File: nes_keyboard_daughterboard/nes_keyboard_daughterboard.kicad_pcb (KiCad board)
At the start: 4 copper layers, 77.2 x 44 mm, 74 parts, among them J1 USB_C_Receptacle_USB2.0_16P, J2 Conn_01x02_Pin, J3 USB_C_Receptacle_USB2.0_16P, U1 NCP1117-3.3_SOT223, U2 USBLC6-2P6

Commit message: Finished V0.1
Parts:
- D1: value White -> Red
- D2: value Orange -> Red
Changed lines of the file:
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@@
 		(sheetname "/")
 		(sheetfile "nes_keyboard_daughterboard.kicad_sch")
+		(units
+			(unit
+				(name "A")
+				(pins "S1" "B1" "B12" "A1" "A12" "A9" "B4" "B9" "A4" "A5" "B5" "A7" "B7"
+					"A6" "B6" "A8" "B8"
+				)
+			)
+		)
 		(attr smd)
 		(duplicate_pad_numbers_are_jumpers no)
@@
 		(sheetname "/")
 		(sheetfile "nes_keyboard_daughterboard.kicad_sch")
+		(units
+			(unit
+				(name "A")
+				(pins "1" "2")
+			)
+		)
 		(attr smd)
 		(duplicate_pad_numbers_are_jumpers no)
@@
 		(sheetname "/")
 		(sheetfile "nes_keyboard_daughterboard.kicad_sch")
+		(units
+			(unit
+				(name "A")
+				(pins "1" "2")
+			)
+		)
 		(attr smd)
 		(duplicate_pad_numbers_are_jumpers no)
@@
 			)
 		)
-		(property "Value" "Orange"
+		(property "Value" "Red"
 			(at 0 1.43 90)
 			(layer "F.Fab")
@@
 		(sheetname "/")
 		(sheetfile "nes_keyboard_daughterboard.kicad_sch")
+		(units
+			(unit
+				(name "A")
+				(pins "1" "2")
+			)
+		)
 		(attr smd)
 		(duplicate_pad_numbers_are_jumpers no)
@@
 		(sheetname "/")
 		(sheetfile "nes_keyboard_daughterboard.kicad_sch")
+		(units
+			(unit
+				(name "A")
+				(pins "1" "2")
+			)
+		)
 		(attr smd)
 		(duplicate_pad_numbers_are_jumpers no)
@@
 			)
 		)
+		(property "Sim.Library" "/home/arya/Downloads/NCP1117 PSPICE MODELS/NCP1117 Model Library.lib"
+			(at 0 0 270)
+			(unlocked yes)
+			(layer "F.Fab")
+			(hide yes)
+			(effects
+				(font
+					(size 1 1)
+					(thickness 0.15)
+				)
+			)
+		)
+		(property "Sim.Name" "ncp1117_33-x"
+			(at 0 0 270)
+			(unlocked yes)
+			(layer "F.Fab")
+			(hide yes)
+			(effects
+				(font
+					(size 1 1)
+					(thickness 0.15)
+				)
+			)
+		)
+		(property "Sim.Device" "SUBCKT"
+			(at 0 0 270)
+			(unlocked yes)
+			(layer "F.Fab")
+			(hide yes)
+			(effects
+				(font
+					(size 1 1)
+					(thickness 0.15)
+				)
+			)
+		)
+		(property "Sim.Pins" "1=1 2=2 3=3"
+			(at 0 0 270)
+			(unlocked yes)
+			(layer "F.Fab")
+			(hide yes)
+			(effects
+				(font
+					(size 1 1)
+					(thickness 0.15)
+				)
+			)
+		)
 		(property ki_fp_filters "SOT?223*TabPin2*")
 		(sheetname "/")
 		(sheetfile "nes_keyboard_daughterboard.kicad_sch")
+		(units
+			(unit
+				(name "A")
+				(pins "3" "1" "2")
+			)
+		)
 		(attr smd)
 		(duplicate_pad_numbers_are_jumpers no)
@@
 			)
 		)
-		(property "Value" "White"
+		(property "Value" "Red"
 			(at 0 1.43 90)
 			(layer "F.Fab")
@@
 			)
 		)
-		(property "Sim.Pins" "1=K 2=A"
+		(property "Sim.Pins" "1=A 2=K"
+			(at 0 0 270)
+			(unlocked yes)
+			(layer "F.Fab")
+			(hide yes)
+			(effects
+				(font
+					(size 1 1)
+					(thickness 0.15)
+				)
+			)
+		)
+		(property "Sim.Device" "D"
+			(at 0 0 270)
+			(unlocked yes)
+			(layer "F.Fab")
+			(hide yes)
+			(effects
+				(font
+					(size 1 1)
+					(thickness 0.15)
+				)
+			)
+		)
+		(property "Sim.Params" "is=0.03 vj=2 bv=5 ibv=0.0001"
 			(at 0 0 270)
 			(unlocked yes)
@@
 		(sheetname "/")
 		(sheetfile "nes_keyboard_daughterboard.kicad_sch")
+		(units
+			(unit
+				(name "A")
+				(pins "1" "2")
+			)
+		)
 		(attr smd)
 		(duplicate_pad_numbers_are_jumpers no)
@@
 		(sheetname "/")
 		(sheetfile "nes_keyboard_daughterboard.kicad_sch")
+		(units
+			(unit
+				(name "A")
+				(pins "1")
+			)
+		)
 		(attr exclude_from_bom)
 		(duplicate_pad_numbers_are_jumpers no)
@@
 		(sheetname "/")
 		(sheetfile "nes_keyboard_daughterboard.kicad_sch")
+		(units
+			(unit
+				(name "A")
+				(pins "1" "3" "5" "2" "6" "4")
+			)
+		)
 		(attr smd)
 		(duplicate_pad_numbers_are_jumpers no)
@@
 		(sheetname "/")
 		(sheetfile "nes_keyboard_daughterboard.kicad_sch")
+		(units
+			(unit
+				(name "A")
+				(pins "1" "2")
+			)
+		)
 		(attr smd)
 		(duplicate_pad_numbers_are_jumpers no)
@@
 		(sheetname "/")
 		(sheetfile "nes_keyboard_daughterboard.kicad_sch")
+		(units
+			(unit
+				(name "A")
+				(pins "S1" "B1" "B12" "A1" "A12" "A9" "B4" "B9" "A4" "A5" "B5" "A7" "B7"
+					"A6" "B6" "A8" "B8"
+				)
+			)
+		)
 		(attr through_hole)
 		(duplicate_pad_numbers_are_jumpers no)
@@
 		(sheetname "/")
 		(sheetfile "nes_keyboard_daughterboard.kicad_sch")
+		(units
+			(unit
+				(name "A")
+				(pins "1" "2")
+			)
+		)
 		(attr smd)
 		(duplicate_pad_numbers_are_jumpers no)
@@
 		(sheetname "/")
 		(sheetfile "nes_keyboard_daughterboard.kicad_sch")
+		(units
+			(unit
+				(name "A")
+				(pins "1")
+			)
+		)
 		(attr exclude_from_bom)
 		(duplicate_pad_numbers_are_jumpers no)
@@
 		(sheetname "/")
 		(sheetfile "nes_keyboard_daughterboard.kicad_sch")
+		(units
+			(unit
+				(name "A")
+				(pins "1" "2")
+			)
+		)
 		(attr through_hole)
 		(duplicate_pad_numbers_are_jumpers no)
@@
 		(sheetname "/")
 		(sheetfile "nes_keyboard_daughterboard.kicad_sch")
+		(units
+			(unit
+				(name "A")
+				(pins "1" "2")
+			)
+		)
 		(attr smd)
 		(duplicate_pad_numbers_are_jumpers no)
@@
 		(sheetname "/")
 		(sheetfile "nes_keyboard_daughterboard.kicad_sch")
+		(units
+			(unit
+				(name "A")
+				(pins "1")
+			)
+		)
 		(attr exclude_from_bom)
 		(duplicate_pad_numbers_are_jumpers no)
@@
 		(sheetname "/")
 		(sheetfile "nes_keyboard_daughterboard.kicad_sch")
+		(units
+			(unit
+				(name "A")
+				(pins "1")
+			)
+		)
 		(attr exclude_from_bom)
 		(duplicate_pad_numbers_are_jumpers no)

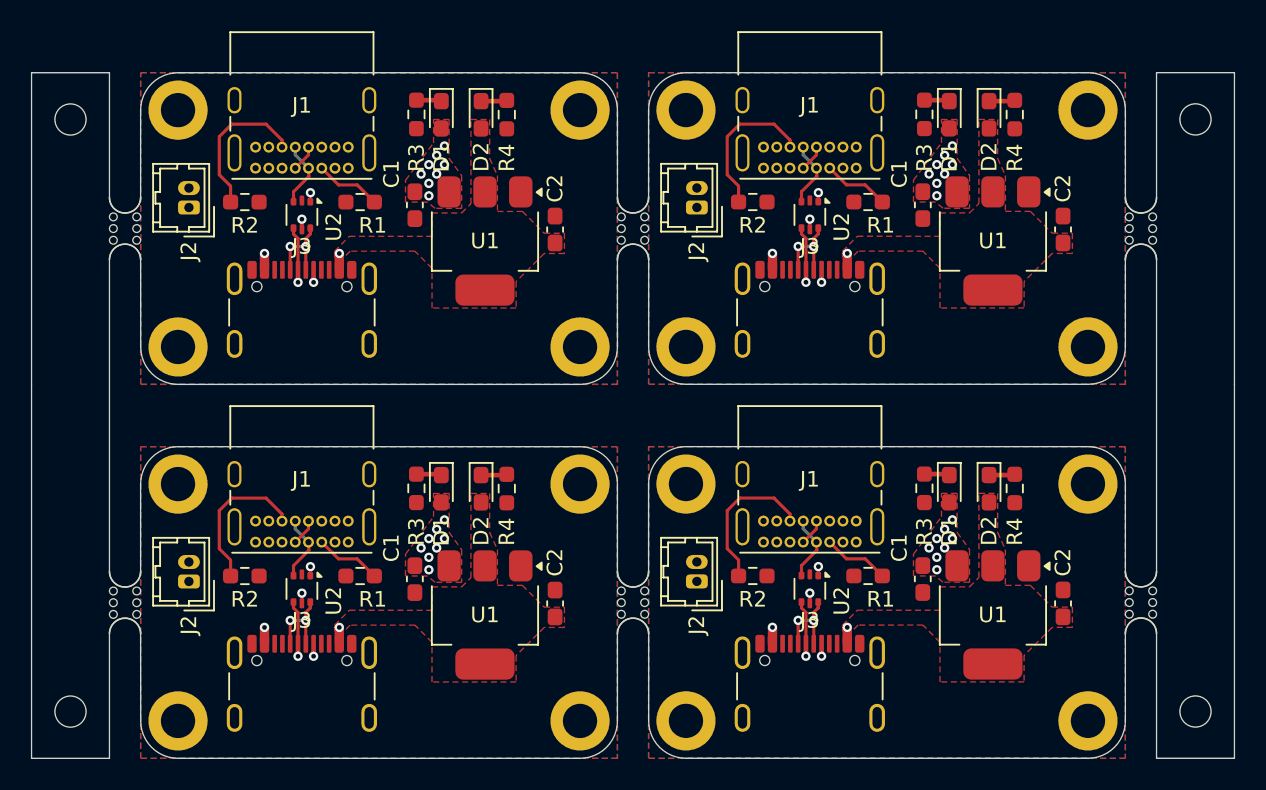
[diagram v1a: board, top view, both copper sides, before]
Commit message: PCB Modifications (all) - V0.2
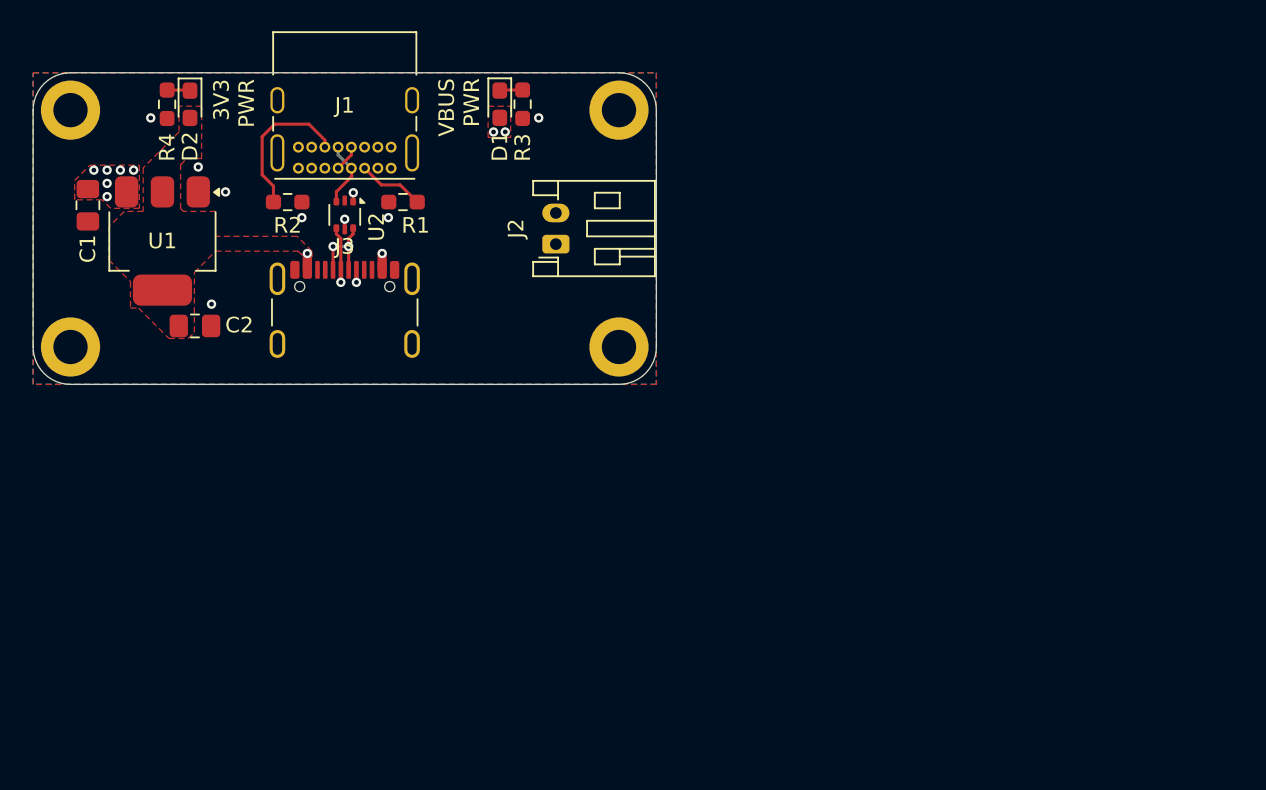
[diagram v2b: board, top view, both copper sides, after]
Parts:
- removed the C1 at (75.1, 28.2)
- removed the C1 at (42.5, 52.2)
- removed the C1 at (75.1, 52.2)
- removed the C1 at (42.5, 28.2)
- removed the C2 at (51.5, 53.8)
- removed the C2 at (84.1, 53.8)
- removed the C2 at (51.5, 29.8)
- removed the C2 at (84.1, 29.8)
- removed the D1 at (76.8, 22.4)
- removed the D1 at (76.8, 46.4)
- removed the D1 at (44.2, 46.4)
- removed the D2 at (46.8, 46.4)
- removed the D2 at (79.4, 22.4)
- removed the D2 at (79.3, 46.4)
- removed the H1 at (27.3, 46.1)
- removed the H1 at (59.9, 22.1)
- removed the H1 at (59.9, 46.1)
- removed the H2 at (59.9, 61.3)
- removed the H2 at (59.9, 37.3)
- removed the H2 at (27.3, 61.3)
- removed the H3 at (85.7, 22.1)
- removed the H3 at (53.1, 46.1)
- removed the H3 at (85.7, 46.1)
- removed the H4 at (85.7, 61.3)
- removed the H4 at (85.7, 37.3)
- removed the H4 at (53.1, 61.3)
- removed the J1 at (70.8, 49.8)
- removed the J1 at (70.8, 25.8)
- removed the J1 at (38.2, 49.8)
- removed the J2 at (28.0, 52.3)
- removed the J2 at (60.6, 52.3)
- removed the J2 at (60.6, 28.3)
- removed the J3 at (67.8, 60.0)
- removed the J3 at (35.2, 60.0)
- removed the J3 at (67.9, 36.0)
- removed the R1 at (71.6, 52.0)
- removed the R1 at (71.6, 28.0)
- removed the R1 at (39.0, 52.0)
- removed the R2 at (64.2, 52.0)
- removed the R2 at (64.2, 28.0)
- removed the R2 at (31.6, 52.0)
- removed the R3 at (42.6, 46.4)
- removed the R3 at (75.2, 46.4)
- removed the R3 at (75.2, 22.4)
- removed the R4 at (81.0, 46.4)
- removed the R4 at (48.4, 46.4)
- removed the R4 at (81.0, 22.4)
- removed the U1 at (79.6, 54.5)
- removed the U1 at (79.6, 30.5)
- removed the U1 at (47.0, 54.5)
- removed the U2 at (67.8, 52.8)
- removed the U2 at (67.9, 28.8)
- removed the U2 at (35.2, 52.8)
- removed mouse-bite-2mm-slot (x6): VAL**, mouse-bite:mouse-bite-2mm-slot
- added C1: 10uF, Capacitor_SMD:C_0805_2012Metric_Pad1.18x1.45mm_HandSolder, F.Cu at (21.5, 28.2)
- added C2: 10uF, Capacitor_SMD:C_0805_2012Metric_Pad1.18x1.45mm_HandSolder, F.Cu at (28.4, 36.0)
- D1: value White -> Red
- D2: value Orange -> Red
- J2: footprint Connector_Hirose:Hirose_DF13-02P-1.25DSA_1x02_P1.25mm_Vertical -> Connector_JST:JST_PH_S2B-PH-K_1x02_P2.00mm_Horizontal
- R3: value 220 -> 680
- R4: value 130 -> 470
- moved J2 23.7 mm to (51.5, 30.7)
- moved R4 21.8 mm to (26.6, 21.7)
- moved U1 20.7 mm to (26.3, 30.5)
- moved D2 18.7 mm to (28.1, 21.7)
- moved H1 6.90 mm to (20.4, 22.1)
- moved H2 6.90 mm to (20.4, 37.3)
- moved R3 6.85 mm to (49.4, 21.7)
- moved D1 3.81 mm to (48.0, 21.7)
- moved J1 2.75 mm to (41.0, 25.8)
- moved J3 2.75 mm to (38.0, 36.0)
- moved R1 2.75 mm to (41.7, 28.0)
- moved R2 2.75 mm to (34.3, 28.0)
- moved U2 2.75 mm to (38.0, 28.8)
- moved H3 2.50 mm to (55.6, 22.1)
- moved H4 2.50 mm to (55.6, 37.3)
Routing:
- net Net-(J1-CC2): track 38.9 -> 9.73 mm
- net +3V3: track 29.9 -> 7.48 mm, vias 8 -> 2
- net /USB_D+: track 22.1 -> 5.52 mm, vias 8 -> 2
- net /USB_D-: track 21.2 -> 5.29 mm, vias 8 -> 2
- net Net-(J1-CC1): track 17.1 -> 4.28 mm
- net /P_USB+: track 17.1 -> 4.27 mm
- net /P_USB-: track 17.0 -> 4.26 mm, vias 4 -> 1
- net Net-(D2-K): track 6.68 -> 1.49 mm
- net Net-(D1-K): track 6.50 -> 1.48 mm
- net VBUS: track 2.60 -> 0.65 mm, vias 36 -> 9
- net GND: vias 0 -> 7
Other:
- board size 77.2 x 44 mm -> 40 x 20 mm
- board text added: "3V3 PWR"
- board text added: "VBUS PWR"
